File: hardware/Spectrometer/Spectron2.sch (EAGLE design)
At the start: 69 parts, among them U1 REF192, U10 ADP7142-2.5, U11 REF195, U12 TLV809, U13 ADG821, U14 ADG3304, U15 LM2662, U16 PHOTON_WITH_HEADERS, U2 ADG1604, U3 ADP7142-5, U4 AD8031, U5 REF193, U6 ADA4841, U7 ADP7142-5, U8 AD7980, U9 REF198

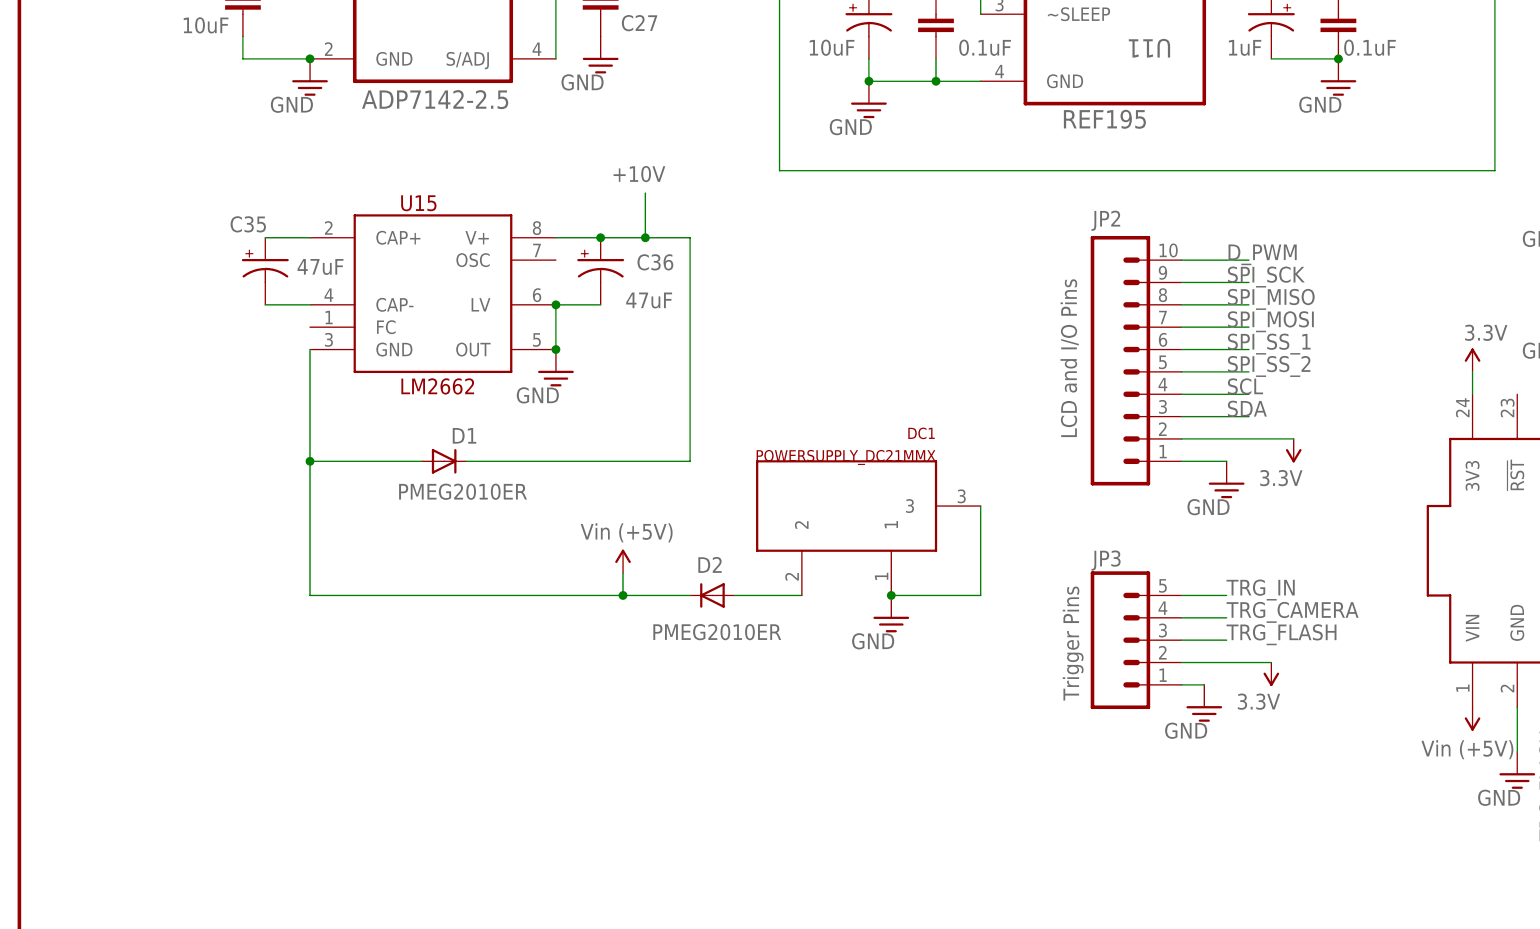
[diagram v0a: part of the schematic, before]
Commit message: Cumulative changes: adding light sources, boards, firmwares, construction details
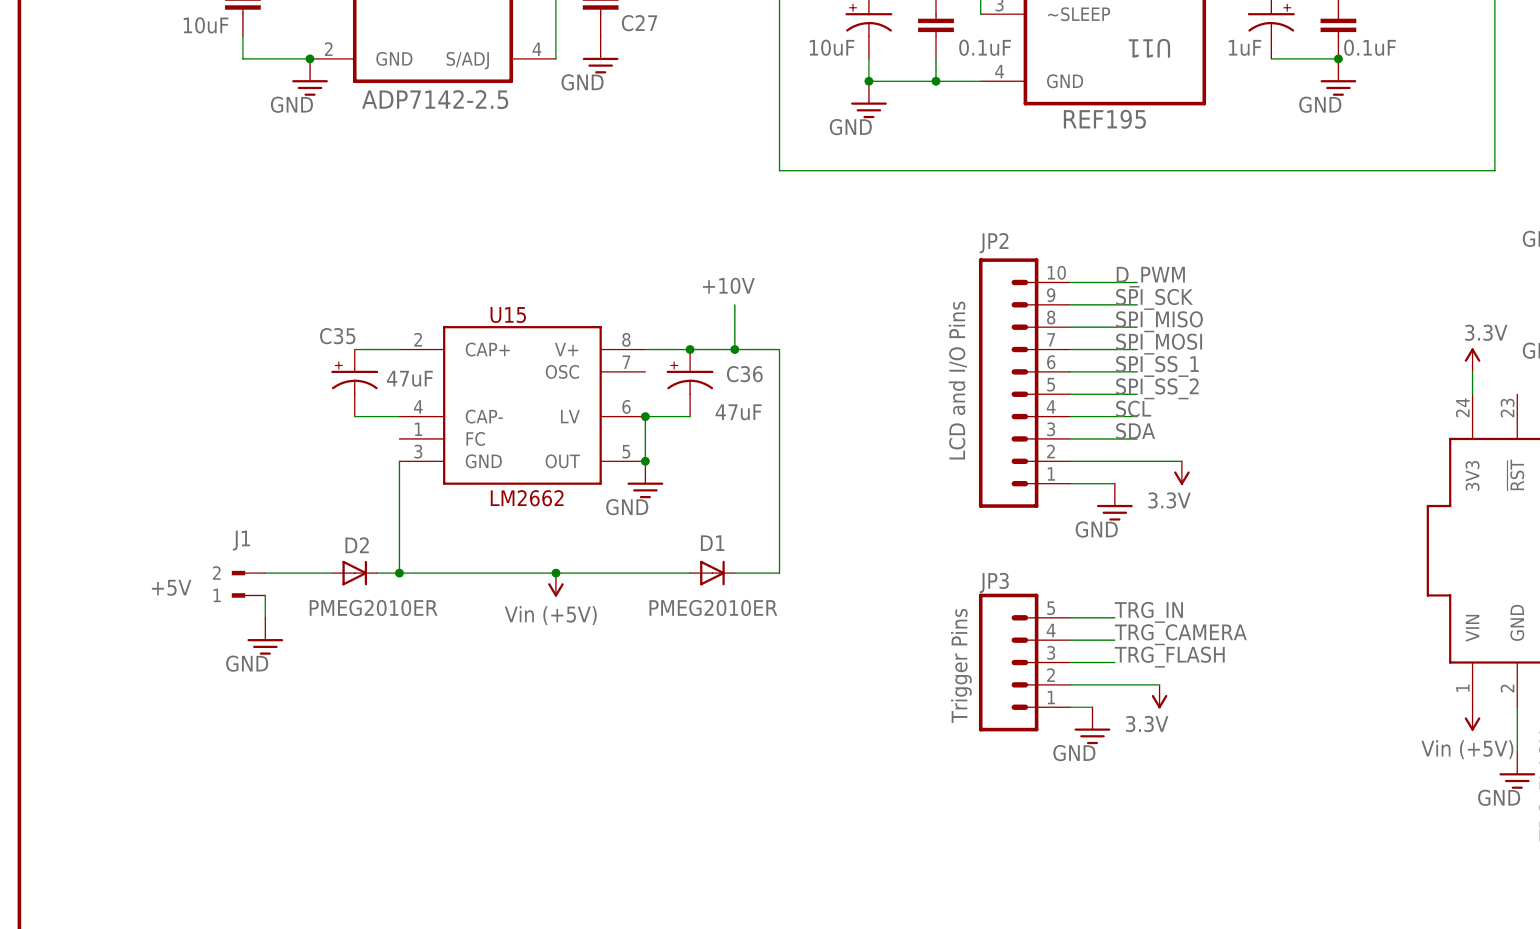
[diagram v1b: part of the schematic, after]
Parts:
- removed DC1: POWERSUPPLY_DC21MMX, Spectron:POWERSUPPLY_DC21MMX
- added J1: +5V, WEIDMULLER-PM5.08_2_90BLK:PM5.08/2/90BLK
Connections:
- net GND: now also J1.1; no longer DC1.1, DC1.3
- net N$11: now also J1.2; no longer DC1.2
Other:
- moved on the sheet: C35, C36, D1, D2, JP2, JP3, U15
